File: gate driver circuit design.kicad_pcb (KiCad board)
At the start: 2 copper layers, 40 x 40 mm, 105 parts, among them J101 90122-0763, J102 90121-0762, J103 90121-0762, Q1 CSD17313Q2, Q2 MMBT3904T-7-F, Q3 MMBT3904T-7-F, Q4 MMBT3904T-7-F, T1 750343725, T2 750343725, U1 SN6501QDBVRQ1, U2 TPS7B6950QDCYRQ1, U3 TL431AQDBZRQ1, U4 SN6501QDBVRQ1, U5 TL431AQDBZRQ1, U6 UCC21530QDWKRQ1, U7 ISO7721QDRQ1, U8 LMV762QMA_NOPB, U9 TL431AQDBZRQ1

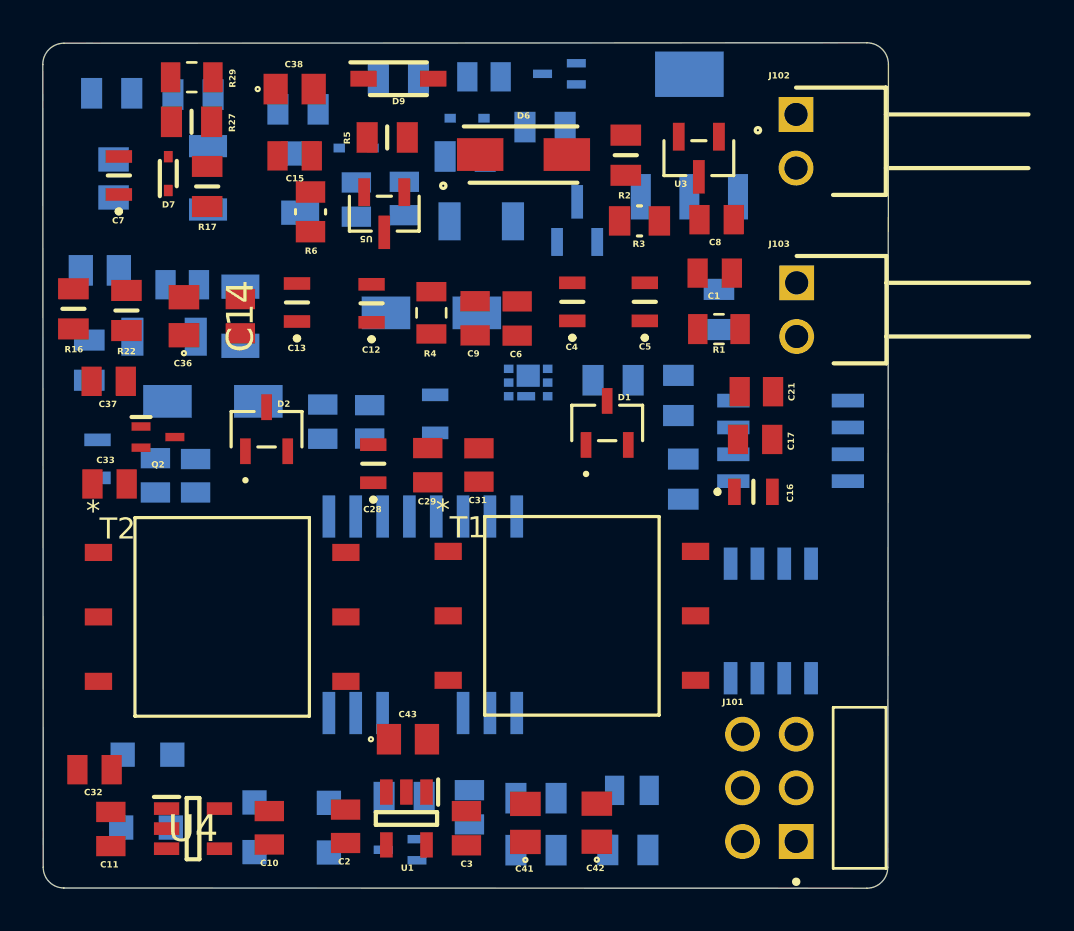
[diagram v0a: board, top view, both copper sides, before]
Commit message: Almost Done Routing Of PCB
Some Connections are remaining , Almost Done Routing Of PCB
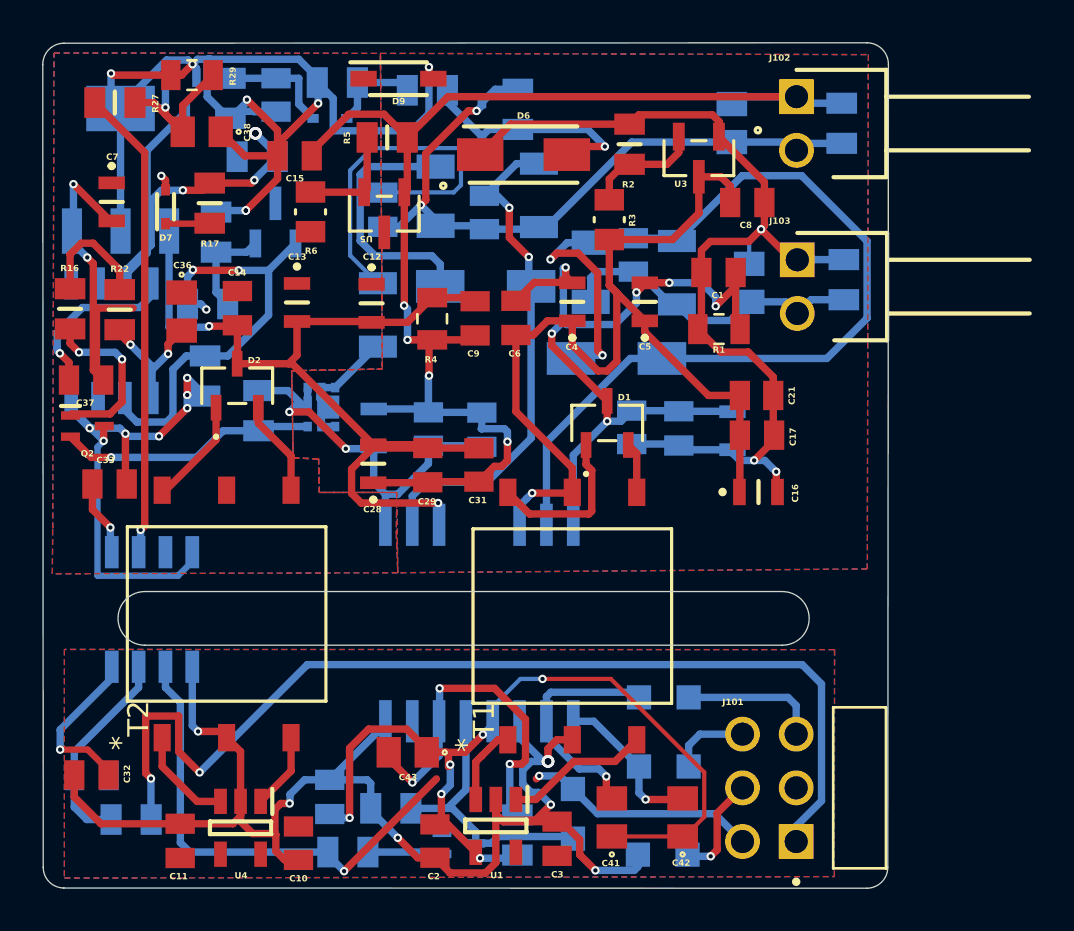
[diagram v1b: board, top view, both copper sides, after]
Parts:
- moved R12 35.9 mm to (115.9, 57.9)
- moved R14 34.6 mm to (115.8, 50.5), turned to -90 degrees
- moved U8 32.5 mm to (81.2, 60.8), turned to -90 degrees
- moved C39 30.7 mm to (111.4, 58.0), turned to 90 degrees
- moved C18 30.1 mm to (110.6, 65.0)
- moved C40 29.4 mm to (110.6, 50.5), turned to 90 degrees
- moved U7 29.3 mm to (83.1, 73.5), turned to 90 degrees
- moved U2 27.0 mm to (81.6, 52.7)
- moved C35 25.6 mm to (80.3, 81.3)
- moved C19 24.9 mm to (108.0, 64.9)
- moved R132 24.5 mm to (107.3, 85.1)
- moved R7 24.5 mm to (108.0, 57.5), turned to -90 degrees
- moved R33 24.4 mm to (107.3, 80.9)
- moved R28 24.1 mm to (86.2, 55.6)
- moved R23 23.6 mm to (82.1, 83.4), turned to 0 degrees
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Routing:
- net -4Vb: track 0.00 -> 90.0 mm, vias 0 -> 11
- net 5Vin: track 0.00 -> 65.4 mm, vias 0 -> 8
- net Comb: track 0.00 -> 62.5 mm, vias 0 -> 4
- net RESET: track 0.00 -> 49.5 mm, vias 0 -> 2
- net GND: track 0.00 -> 49.5 mm, vias 0 -> 7
- net Coma: track 0.00 -> 49.0 mm, vias 0 -> 3
- net -4Va: track 0.00 -> 47.2 mm, vias 0 -> 1
- net Vcc5V: track 0.00 -> 45.4 mm, vias 0 -> 9
- net +15Vb: track 0.00 -> 44.4 mm, vias 0 -> 2
- net Net-(D3-K): track 0.00 -> 38.8 mm
- net +15Va: track 0.00 -> 38.2 mm, vias 0 -> 6
- net FLT: track 0.00 -> 33.7 mm, vias 0 -> 2
- net G2: track 0.00 -> 33.0 mm, vias 0 -> 2
- net Net-(D4-K): track 0.00 -> 24.1 mm, vias 0 -> 2
- net Net-(U7-OUTB): track 0.00 -> 22.9 mm, vias 0 -> 1
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- added copper zone on B.Cu, net (none)
- added copper zone on F.Cu, net (none)
- added copper zone on B.Cu, net -4Vb
- added copper zone on F.Cu, net -4Vb
- added copper zone on B.Cu, net GND
- added copper zone on F.Cu, net GND
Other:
- outline, holes or cut-outs redrawn
